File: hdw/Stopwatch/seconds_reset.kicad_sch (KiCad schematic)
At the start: 9 parts

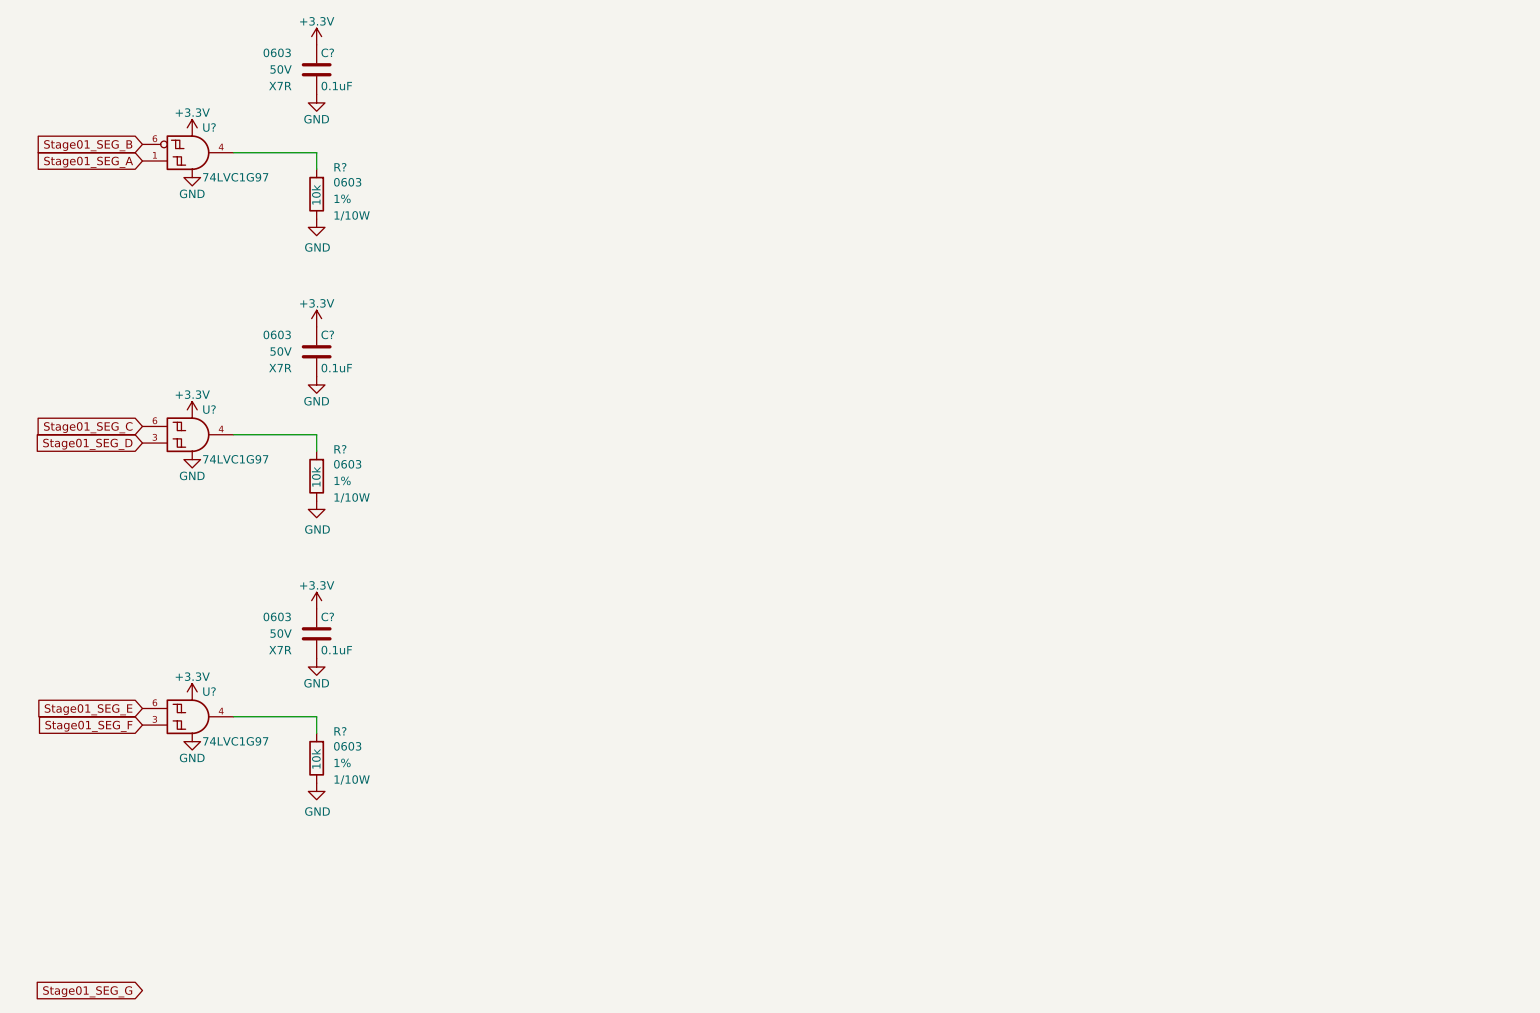
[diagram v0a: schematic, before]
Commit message: added more reset stuff
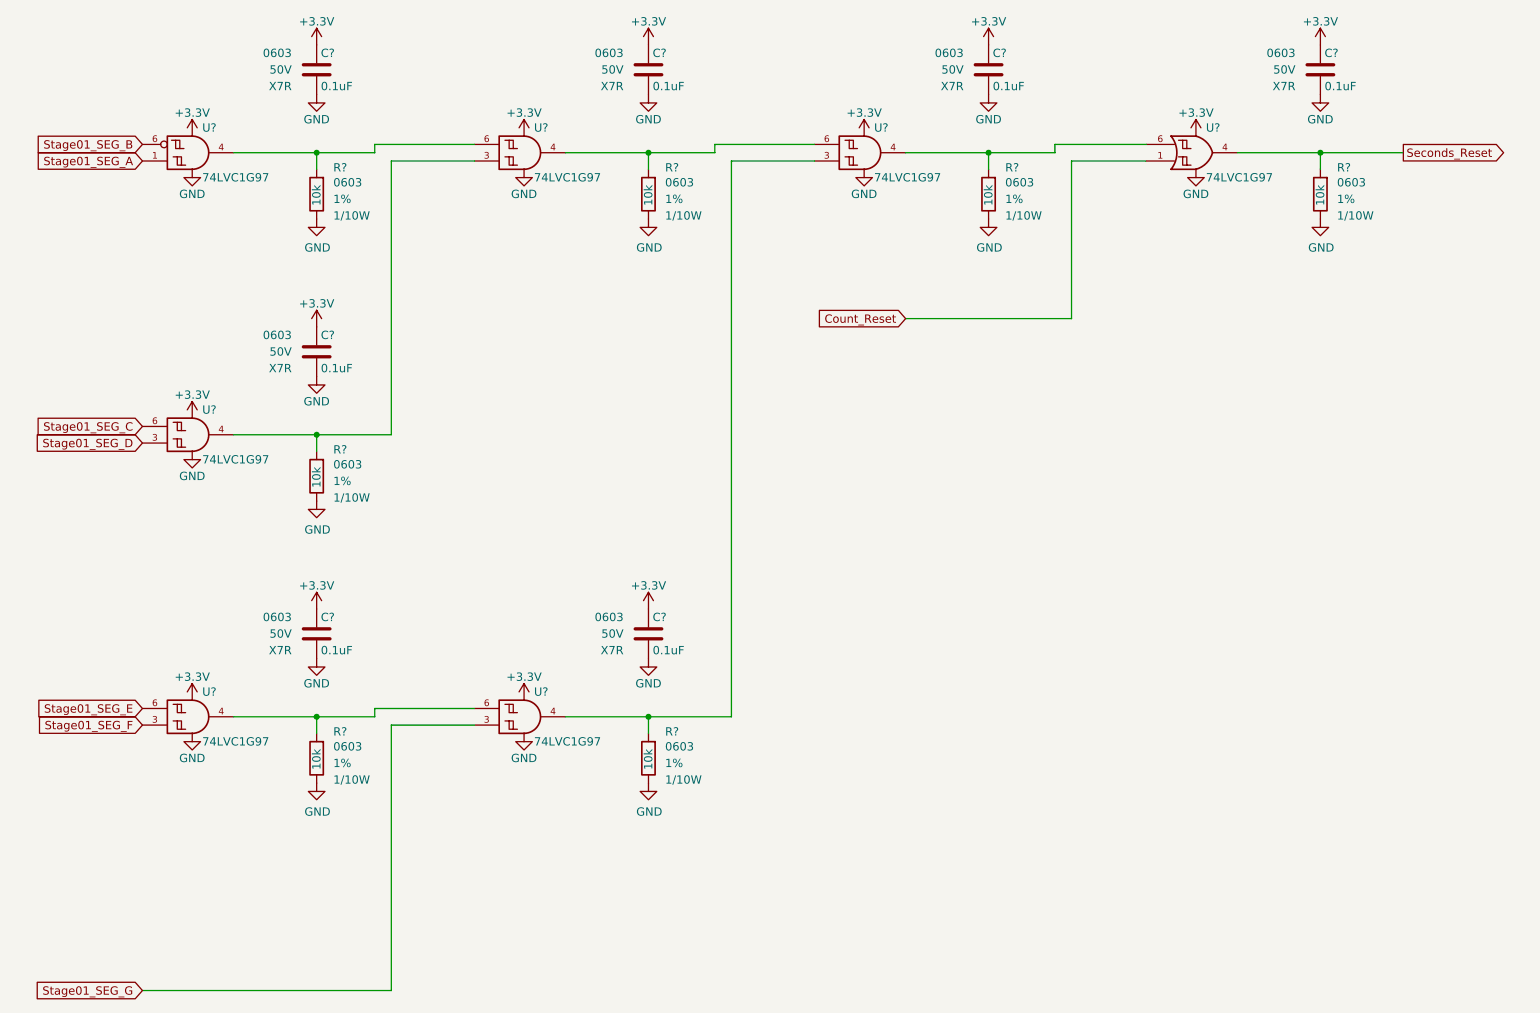
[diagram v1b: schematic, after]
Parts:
- added C? (x4): 0.1uF, Capacitors_SMD:C_0603, symbol Custom_Library:C_Custom
- added R? (x4): 10k, Resistors_SMD:R_0603, symbol Custom_Library:R_Custom
- added U?: 74LVC1G97, Package_TO_SOT_SMD:SOT-363_SC-70-6, symbol Custom Library:74LVC1G97_Power_OR
- added U? (x3): 74LVC1G97, Package_TO_SOT_SMD:SOT-363_SC-70-6, symbol Custom Library:74LVC1G97_Power_AND
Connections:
- net +3.3V: now also U?.3 (VCC), U?.5 (VCC), U?.5 (VCC), U?.5 (VCC), U?.5 (VCC)
- net +3V3: now also C?.1, C?.1, C?.1, C?.1
- net GND: now also C?.2, C?.2, C?.2, C?.2, R?.2, R?.2, R?.2, R?.2, U?.1 (GND), U?.1 (GND), U?.1 (GND), U?.2 (GND), U?.2 (GND), U?.2 (GND), U?.2 (GND)
- net Stage01_SEG_G: now also U?.3
- net at R?.1, U?.4: now also U?.3
- net at R?.1, U?.4: now also U?.6 (x2)
- new net: R?.1, U?.4, U?.6 (x2)
- new net: R?.1, U?.3, U?.4
- new net Count_Reset: U?.1
- new net Seconds_Reset: R?.1, U?.4
